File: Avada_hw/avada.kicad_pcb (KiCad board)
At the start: 2 copper layers, 30.2 x 53.5 mm, 40 parts, among them Q1 IRLML6401, Q2 IRLML6401, Q3 NSS20101, Q4 NSS20101, Q5 NSS20101, SW1 IT1198, SW2 DIPx6, SW3 SS-1P2T

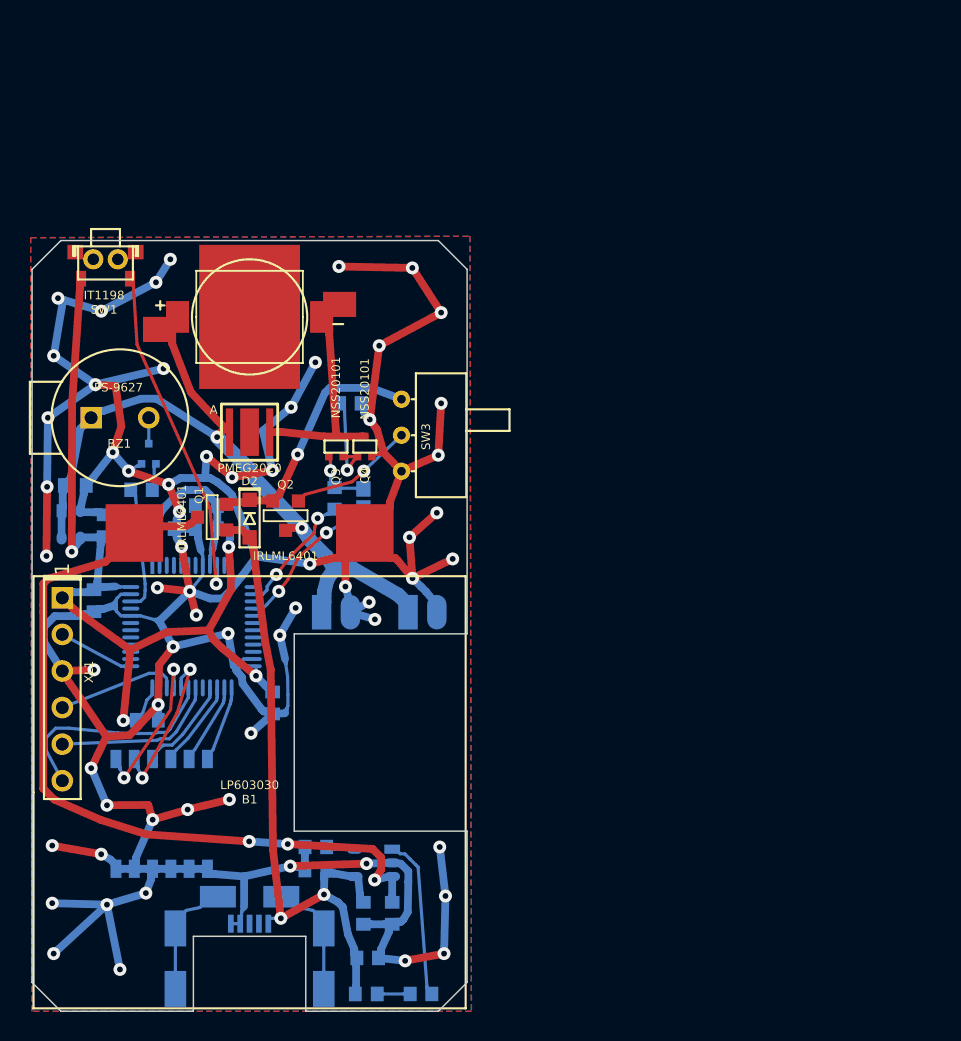
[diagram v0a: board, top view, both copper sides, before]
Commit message: Some renamings
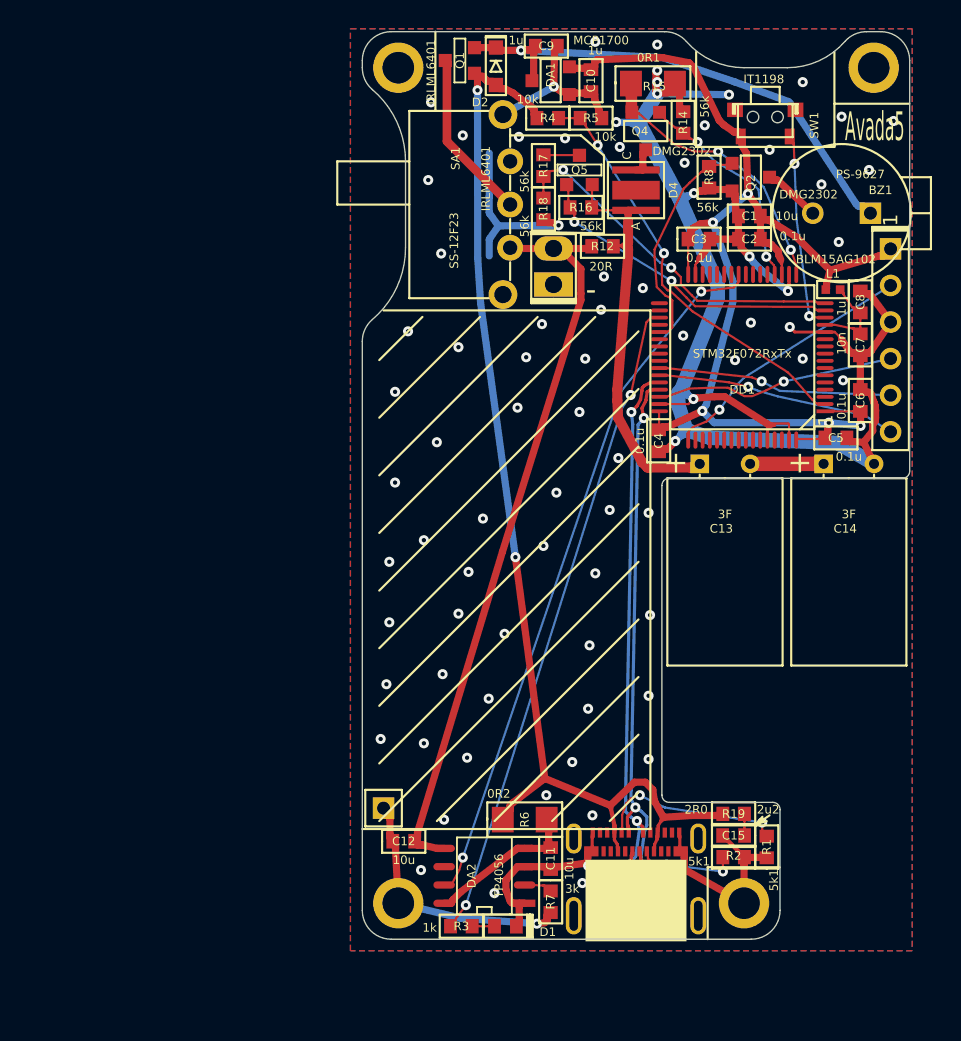
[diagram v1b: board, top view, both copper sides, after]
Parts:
- removed B1: LP603030, Installation:EEMB603030
- removed D3: LED, LEDs:LED_Diamond_Dragon
- removed D5: LED, LEDs:LED_XPE
- removed F1: Fuse0R, Resistors:RES_0603_FUSE
- removed Q3: NSS20101, SOT:SC89-3
- removed SW2: DIPx6, BtnsSwitches:DIP_SMD_1D27X6
- removed SW3: SS-1P2T, BtnsSwitches:SW_SS-1P2T_R
- added C14: 3F, Capacitors:CAP_08xxR_HOR, F.Cu at (160.6, 86.2)
- added C15: 2u2, Capacitors:CAP_0603_Silks, F.Cu at (152.6, 112.0)
- added HOLE1: HOLE_METALLED, PCB:Hole2d2_out3d5mm, F.Cu at (153.3, 116.7)
- added HOLE2: HOLE_METALLED, PCB:Hole2d2_out3d5mm, F.Cu at (129.3, 58.7)
- added HOLE3: HOLE_METALLED, PCB:Hole2d2_out3d5mm, F.Cu at (129.3, 116.7)
- added HOLE4: HOLE_METALLED, PCB:Hole2d2_out3d5mm, F.Cu at (162.3, 58.7)
- added L1: BLM15AG102, Inductors:IND_0402, F.Cu at (159.5, 74.1)
- added R12: 20R, Resistors:RES_0603, F.Cu at (143.5, 71.1)
- added R14: 56k, Resistors:RES_0603, F.Cu at (149.1, 62.5)
- added R15: 0R1, Resistors:RES_1206, F.Cu at (147.0, 59.8)
- added R16: 56k, Resistors:RES_0603, F.Cu at (142.0, 68.4)
- added R17: 56k, Resistors:RES_0603, F.Cu at (139.4, 65.5)
- added R18: 56k, Resistors:RES_0603, F.Cu at (139.4, 68.5)
- added R19: 2R0, Resistors:RES_0603, F.Cu at (152.6, 110.5)
- added R7: 3k, Resistors:RES_0603, F.Cu at (139.9, 116.6)
- added R8: 56k, Resistors:RES_0603, F.Cu at (150.9, 66.3)
- added SA1: SS-12F23, BtnsSwitches:SW_SS-12F23, F.Cu at (137.1, 68.2)
- added XL3: USB_C, Connectors:USB_C_MOLEX_1054500101, F.Cu at (145.8, 119.3)
- added XL4: CONN_1, Connectors:PLS-1Square, F.Cu at (128.3, 110.1)
- C1: value 10n -> 10u; footprint Capacitors:CAP_0603 -> Capacitors:CAP_0603_Silks; moved to F.Cu
- C10: value 10n -> 1u; footprint Capacitors:CAP_0603 -> Capacitors:CAP_0603_Silks; moved to F.Cu
- C11: value 1u -> 10u; footprint Capacitors:CAP_0603 -> Capacitors:CAP_0603_Silks; moved to F.Cu
- C12: value 220u -> 10u; footprint Capacitors:CAP_05xxR_horiz_HOLE -> Capacitors:CAP_0603_Silks; moved to F.Cu
- C13: value 220u -> 3F; footprint Capacitors:CAP_05xxR_horiz_HOLE -> Capacitors:CAP_08xxR_HOR; moved to F.Cu
- C2, C4, C6: value 10u -> 0.1u; footprint Capacitors:CAP_0603 -> Capacitors:CAP_0603_Silks; moved to F.Cu
- C3, C5: value 1u -> 0.1u; footprint Capacitors:CAP_0603 -> Capacitors:CAP_0603_Silks; moved to F.Cu
- C7: value 0.1u -> 10n; footprint Capacitors:CAP_0603 -> Capacitors:CAP_0603_Silks; moved to F.Cu
- C8, C9: value 0.1u -> 1u; footprint Capacitors:CAP_0603 -> Capacitors:CAP_0603_Silks; moved to F.Cu
- D1: value LED -> L-C191LBCT; moved to F.Cu
- D4: value LED -> LEDwPAD; footprint LEDs:LED_RAD -> LEDs:LED_XPE
- DA1: value MCP73832 -> MCP1700; footprint SOT:SOT23-5 -> SOT:SOT23-3A; moved to F.Cu
- DA2: value NCP583SQ -> TP4056; footprint SOT:SC82AB -> SO_DIL_TSSOP:SO8_150MIL; moved to F.Cu
- DD1: value STM32L151CxTx -> STM32F072RxTx; footprint LQFP_TQFP:LQFP48 -> LQFP_TQFP:LQFP64; moved to F.Cu
- Q2: value IRLML6401 -> DMG2302; footprint SOT:SOT23-3 -> SOT:SOT23-3A
- Q4: value NSS20101 -> DMG2302; footprint SOT:SC89-3 -> SOT:SOT23-3A
- Q5: value NSS20101 -> IRLML6401; footprint SOT:SC89-3 -> SOT:SOT23-3; moved to F.Cu
- R1: value 1k -> 5k1; moved to F.Cu
- R2: value 3k -> 5k1; moved to F.Cu
- R3: value 10k -> 1k; moved to F.Cu
- R4: moved to F.Cu
- R5: value 1k -> 10k; moved to F.Cu
- R6: value 1k -> 0R2; footprint Resistors:RES_0603 -> Resistors:RES_1206; moved to F.Cu
- XL2: value USB_Micro_B -> CONN_2; footprint Connectors:USBmicro_MOLEX_WM17142 -> Connectors:SLD_2_2D5; moved to F.Cu
- moved XL1 62.4 mm to (163.5, 71.3)
- moved C8 57.4 mm to (161.4, 75.0), turned to 90 degrees
- moved DA1 55.7 mm to (139.9, 59.6)
- moved C1 54.5 mm to (153.7, 69.0), turned to 180 degrees
- moved C2 53.9 mm to (153.7, 70.6), turned to 180 degrees
- moved BZ1 52.1 mm to (160.1, 68.8), turned to 0 degrees
- moved C5 51.2 mm to (159.7, 84.4), turned to 0 degrees
- moved XL2 51.1 mm to (140.1, 72.5)
- moved C9 49.7 mm to (139.6, 57.2), turned to 0 degrees
- moved C7 47.8 mm to (161.4, 77.9)
- moved SW1 47.3 mm to (154.8, 60.0)
- moved C3 46.6 mm to (150.2, 70.6)
- moved C6 46.0 mm to (161.4, 81.8), turned to 90 degrees
- moved C10 43.0 mm to (142.7, 59.6), turned to -90 degrees
- moved DD1 42.5 mm to (153.2, 78.8), turned to 180 degrees
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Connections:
- net /LED_OUT renamed Net-(D4-PadC)
- BZ1 pad 1: PwrUnst -> +PwrUnst
- C1 pad 1: GND -> +PwrMCU
- C1 pad 2: +5V -> GND
- C10 pad 1: PwrMCU -> +PwrMCU
- C11 pad 1: PwrMCU -> GND
- C11 pad 2: GND -> /5V_MID
- C12 pad 1: PwrUnst -> GND
- C12 pad 2: GND -> +BATT
- C13 pad 1: PwrUnst -> Net-(C13-Pad1)
- C13 pad 2: GND -> Net-(C13-Pad2)
- C2 pad 1: GND -> +PwrMCU
- C2 pad 2: +5V -> GND
- C3 pad 1: PwrUnst -> +PwrMCU
- C4 pad 1: GND -> +PwrMCU
- C4 pad 2: +BATT -> GND
- C5 pad 1: PwrMCU -> +PwrMCU
- C6 pad 1: GND -> +PwrMCU
- C6 pad 2: PwrMCU -> GND
- C7 pad 1: PwrMCU -> Net-(C7-Pad1)
- C8 pad 1: PwrMCU -> Net-(C7-Pad1)
- C9 pad 1: PwrMCU -> +PwrUnst
- D1 pad A: +5V -> Net-(D1-PadA)
- D1 pad C: Net-(D1-PadC) -> GND
- D2 pad A: +5V -> /+5V_USB
- D2 pad C: /PWR_ALWAYS -> +PwrUnst
- D4 pad A: PwrUnst -> Net-(C13-Pad1)
- DA1 pad 1: /Charge -> GND
- DA1 pad 2: GND -> +PwrMCU
- DA1 pad 3: +BATT -> +PwrUnst
- DA2 pad 1: PwrUnst -> GND
- DA2 pad 2: GND -> Net-(DA2-Pad2)
- DA2 pad 3: PwrMCU -> GND
- DA2 pad 4: PwrUnst -> /5V_MID
- DD1 pad 1: PwrMCU -> +PwrMCU
- DD1 pad 10: Net-(DD1-Pad10) -> unconnected-(DD1-Pad10)
- DD1 pad 11: (no net) -> unconnected-(DD1-Pad11)
- DD1 pad 12: (no net) -> GND
- DD1 pad 13: (no net) -> Net-(C7-Pad1)
- DD1 pad 14: /LED_DAC -> Net-(DD1-Pad14)
- DD1 pad 15: (no net) -> /MeasEn
- DD1 pad 16: /LED_TIM -> /LED_V
- DD1 pad 17: (no net) -> /LED_CURR
- DD1 pad 18: (no net) -> GND
- DD1 pad 19: (no net) -> +PwrMCU
- DD1 pad 2: (no net) -> /USB_DETECT
- DD1 pad 20: (no net) -> /LED_CTRL
- DD1 pad 21: (no net) -> unconnected-(DD1-Pad21)
- DD1 pad 22: (no net) -> unconnected-(DD1-Pad22)
- DD1 pad 23: GND -> unconnected-(DD1-Pad23)
- DD1 pad 24: PwrMCU -> unconnected-(DD1-Pad24)
- DD1 pad 25: /DS1 -> /IS_CHARGING
- DD1 pad 26: /DS2 -> unconnected-(DD1-Pad26)
- DD1 pad 27: /DS3 -> unconnected-(DD1-Pad27)
- DD1 pad 28: /DS4 -> unconnected-(DD1-Pad28)
- DD1 pad 29: (no net) -> unconnected-(DD1-Pad29)
- DD1 pad 3: (no net) -> unconnected-(DD1-Pad3)
- DD1 pad 30: /UART_TX -> unconnected-(DD1-Pad30)
- DD1 pad 31: /UART_RX -> GND
- DD1 pad 32: /DS5 -> +PwrMCU
- DD1 pad 33: /DS6 -> unconnected-(DD1-Pad33)
- DD1 pad 34: /SWDIO -> unconnected-(DD1-Pad34)
- DD1 pad 35: GND -> Net-(DD1-Pad35)
- DD1 pad 36: PwrMCU -> unconnected-(DD1-Pad36)
- DD1 pad 37: /SWCLK -> /Buzzer
- DD1 pad 38: (no net) -> unconnected-(DD1-Pad38)
- DD1 pad 39: (no net) -> unconnected-(DD1-Pad39)
- DD1 pad 4: (no net) -> unconnected-(DD1-Pad4)
- DD1 pad 40: (no net) -> unconnected-(DD1-Pad40)
- DD1 pad 41: (no net) -> unconnected-(DD1-Pad41)
- DD1 pad 42: (no net) -> /UART_TX
- DD1 pad 43: (no net) -> /UART_RX
- DD1 pad 44: GND -> /USB_D-
- DD1 pad 45: (no net) -> /USB_D+
- DD1 pad 46: /Buzzer -> /SWDIO
- DD1 pad 48: PwrMCU -> +PwrMCU
- DD1 pad 5: (no net) -> unconnected-(DD1-Pad5)
- DD1 pad 6: (no net) -> unconnected-(DD1-Pad6)
- DD1 pad 7: (no net) -> unconnected-(DD1-Pad7)
- DD1 pad 8: GND -> unconnected-(DD1-Pad8)
- DD1 pad 9: PwrMCU -> unconnected-(DD1-Pad9)
- Q1 pad 1: +5V -> /+5V_USB
- Q1 pad 2: /PWR_ALWAYS -> +PwrUnst
- Q1 pad 3: +BATT -> Net-(Q1-Pad3)
- Q2 pad 1: Net-(Q2-Pad1) -> /Buzzer
- Q2 pad 2: /PWR_ALWAYS -> GND
- Q2 pad 3: PwrUnst -> /BuzzerOut
- Q4 pad 1: Net-(Q3-Pad2) -> /LED_CTRL
- Q4 pad 2: GND -> /LED_CURR
- Q5 pad 1: Net-(Q5-Pad1) -> /MeasEn
- Q5 pad 2: GND -> Net-(C13-Pad1)
- Q5 pad 3: /BuzzerOut -> Net-(Q5-Pad3)
- R1 pad 1: /Charge -> GND
- R1 pad 2: Net-(D1-PadC) -> Net-(R1-Pad2)
- R2 pad 1: Net-(DA1-Pad5) -> GND
- R2 pad 2: GND -> Net-(R2-Pad2)
- R3 pad 1: +5V -> Net-(D1-PadA)
- R3 pad 2: GND -> Net-(DD1-Pad35)
- R4 pad 1: Net-(F1-Pad1) -> /+5V_USB
- R4 pad 2: /LED_DAC -> /USB_DETECT
- R5 pad 1: Net-(Q3-Pad2) -> /USB_DETECT
- R6 pad 1: /Buzzer -> /+5V_USB
- R6 pad 2: Net-(Q5-Pad1) -> /5V_MID
- SW1 pad 1: Net-(DD1-Pad10) -> Net-(DD1-Pad14)
- SW1 pad 2: PwrMCU -> +PwrMCU
- SW1 pad H: (no net) -> GND
- XL1 pad 1: PwrMCU -> +PwrMCU
- XL2 pad 1: +5V -> GND
- XL2 pad 2: (no net) -> +BATT
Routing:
- net GND: track 332.0 -> 193.3 mm, vias 63 -> 84
- net +PwrMCU: track 0.00 -> 83.2 mm, vias 0 -> 5
- net /+5V_USB: track 0.00 -> 81.1 mm, vias 0 -> 2
- net PwrMCU: track 80.7 -> 0.00 mm, vias 4 -> 0
- net PwrUnst: track 51.6 -> 0.00 mm, vias 2 -> 0
- net /IS_CHARGING: track 0.00 -> 49.0 mm, vias 0 -> 2
- net +5V: track 46.8 -> 0.00 mm, vias 2 -> 0
- net Net-(DD1-Pad35): track 0.00 -> 45.3 mm, vias 0 -> 2
- net /USB_D+: track 0.00 -> 37.8 mm, vias 0 -> 3
- net /USB_D-: track 0.00 -> 37.1 mm, vias 0 -> 3
- net +PwrUnst: track 0.00 -> 35.8 mm, vias 0 -> 1
- net Net-(C13-Pad1): track 0.00 -> 29.3 mm
- net /USB_DETECT: track 0.00 -> 29.0 mm, vias 0 -> 2
- net /LED_V: track 0.00 -> 25.1 mm, vias 0 -> 2
- net Net-(DD1-Pad10): track 23.6 -> 0.00 mm, vias 1 -> 0
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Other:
- board size 30.2 x 53.5 mm -> 38 x 63 mm
- net class Default removed
- net class Wide removed
- rule pad_to_mask_clearance: 0.1 -> 0.06
- board text added: "-"
- board text added: "Avada5"
